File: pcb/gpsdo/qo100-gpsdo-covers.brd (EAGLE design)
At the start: 75 x 79 mm, 1 part

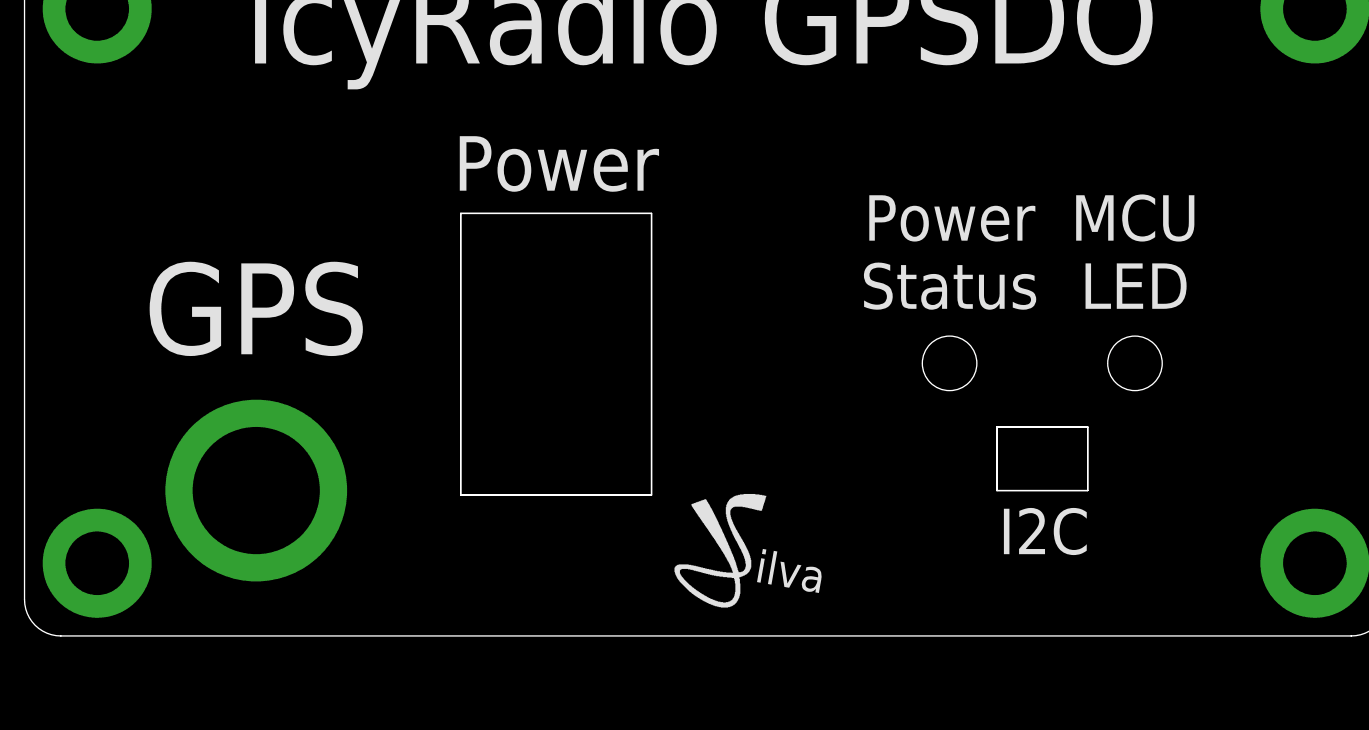
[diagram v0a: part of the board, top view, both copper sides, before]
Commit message: Update GPSDO covers
Signed-off-by: João Silva <jgc3silva@gmail.com>
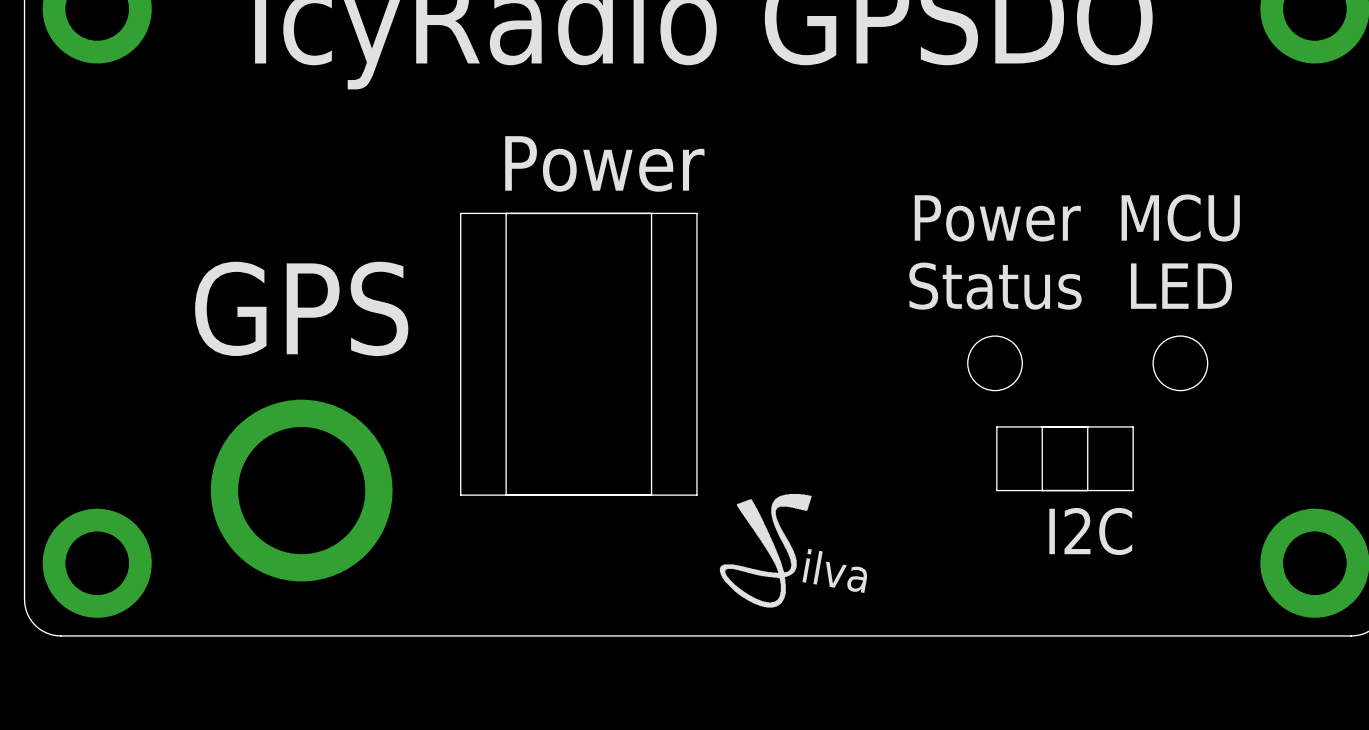
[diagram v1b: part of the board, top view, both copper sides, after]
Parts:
- moved E$1 2.50 mm to (43.5, 8.00)
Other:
- outline, holes or cut-outs redrawn
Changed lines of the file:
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@@
 <drawing>
 <settings>
-<setting alwaysvectorfont="yes"/>
+<setting alwaysvectorfont="no"/>
 <setting verticaltext="up"/>
 </settings>
-<grid distance="1" unitdist="mm" unit="mm" style="lines" multiple="1" display="yes" altdistance="0.1" altunitdist="mm" altunit="mm"/>
+<grid distance="2.5" unitdist="mm" unit="mm" style="lines" multiple="1" display="yes" altdistance="0.1" altunitdist="mm" altunit="mm"/>
 <layers>
 <layer number="1" name="Top" color="4" fill="1" visible="yes" active="yes"/>
@@
 <wire x1="35" y1="38.5" x2="2" y2="38.5" width="0" layer="20"/>
 <wire x1="2" y1="38.5" x2="0" y2="36.5" width="0" layer="20" curve="90"/>
-<rectangle x1="24" y1="7.75" x2="34.5" y2="23.25" layer="20"/>
-<rectangle x1="53.5" y1="8" x2="58.5" y2="11.5" layer="20"/>
-<hole x="50.9" y="15" drill="3"/>
-<hole x="61.1" y="15" drill="3"/>
+<rectangle x1="26.5" y1="7.75" x2="37" y2="23.25" layer="20"/>
+<rectangle x1="56" y1="8" x2="61" y2="11.5" layer="20"/>
+<hole x="53.4" y="15" drill="3"/>
+<hole x="63.6" y="15" drill="3"/>
 <rectangle x1="35" y1="38.3" x2="37.25" y2="40.7" layer="41"/>
 <rectangle x1="37.75" y1="38.3" x2="40" y2="40.7" layer="41"/>
@@
 <wire x1="1.8" y1="57.5" x2="3.8" y2="57.5" width="0.4" layer="21" curve="-141.419908"/>
 <wire x1="6.2" y1="55.5" x2="4.2" y2="55.5" width="0.4" layer="21" curve="-141.419908"/>
-<text x="50.9" y="18" size="2.5" layer="21" font="vector" ratio="13" align="bottom-center">Power
+<text x="53.4" y="18" size="2.5" layer="21" font="vector" ratio="13" align="bottom-center">Power
 Status</text>
-<text x="12.75" y="18" size="5" layer="21" font="vector" ratio="14" rot="R180" align="center">GPS</text>
-<text x="29.25" y="26" size="3" layer="21" font="vector" ratio="14" rot="R180" align="center">Power</text>
-<text x="61.1" y="18" size="2.5" layer="21" font="vector" ratio="13" align="bottom-center">MCU
+<text x="15.25" y="18" size="5" layer="21" font="vector" ratio="14" rot="R180" align="center">GPS</text>
+<text x="31.75" y="26" size="3" layer="21" font="vector" ratio="14" rot="R180" align="center">Power</text>
+<text x="63.6" y="18" size="2.5" layer="21" font="vector" ratio="13" align="bottom-center">MCU
 LED</text>
-<text x="56.1" y="7" size="2.5" layer="21" font="vector" ratio="13" align="top-center">I2C</text>
+<text x="58.6" y="7" size="2.5" layer="21" font="vector" ratio="13" align="top-center">I2C</text>
 <text x="37.25" y="34" size="5" layer="21" font="vector" ratio="14" rot="R180" align="center">IcyRadio GPSDO</text>
 <rectangle x1="24" y1="7.75" x2="34.5" y2="23.25" layer="46"/>
@@
 </autorouter>
 <elements>
-<element name="E$1" library="Silkscreen" package="JSILVA_5MM" value="" x="41" y="8" smashed="yes"/>
+<element name="E$1" library="Silkscreen" package="JSILVA_5MM" value="" x="43.5" y="8" smashed="yes"/>
 </elements>
 <signals>
@@
 <vertex x="-10" y="90"/>
 </polygon>
-<via x="12.75" y="8" extent="1-16" drill="7" diameter="10" alwaysstop="yes"/>
+<via x="15.25" y="8" extent="1-16" drill="7" diameter="10" alwaysstop="yes"/>
 <via x="4" y="75" extent="1-16" drill="3.5" diameter="6" alwaysstop="yes"/>
 <via x="4" y="44.5" extent="1-16" drill="3.5" diameter="6" alwaysstop="yes"/>
